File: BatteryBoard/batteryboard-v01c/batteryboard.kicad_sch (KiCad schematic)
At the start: 29 parts, among them J1 KEYSTONE-1042, J2 KEYSTONE-1042, J3 KEYSTONE-1042, J4 KEYSTONE-1042, J5 KEYSTONE-1042, J6 KEYSTONE-1042, J7 5023520601, J8 Screw_Terminal_01x02, Q1 IRF7458, Q2 IRF7458, Q3 MMBT2222AT, U1 R5460N233AF

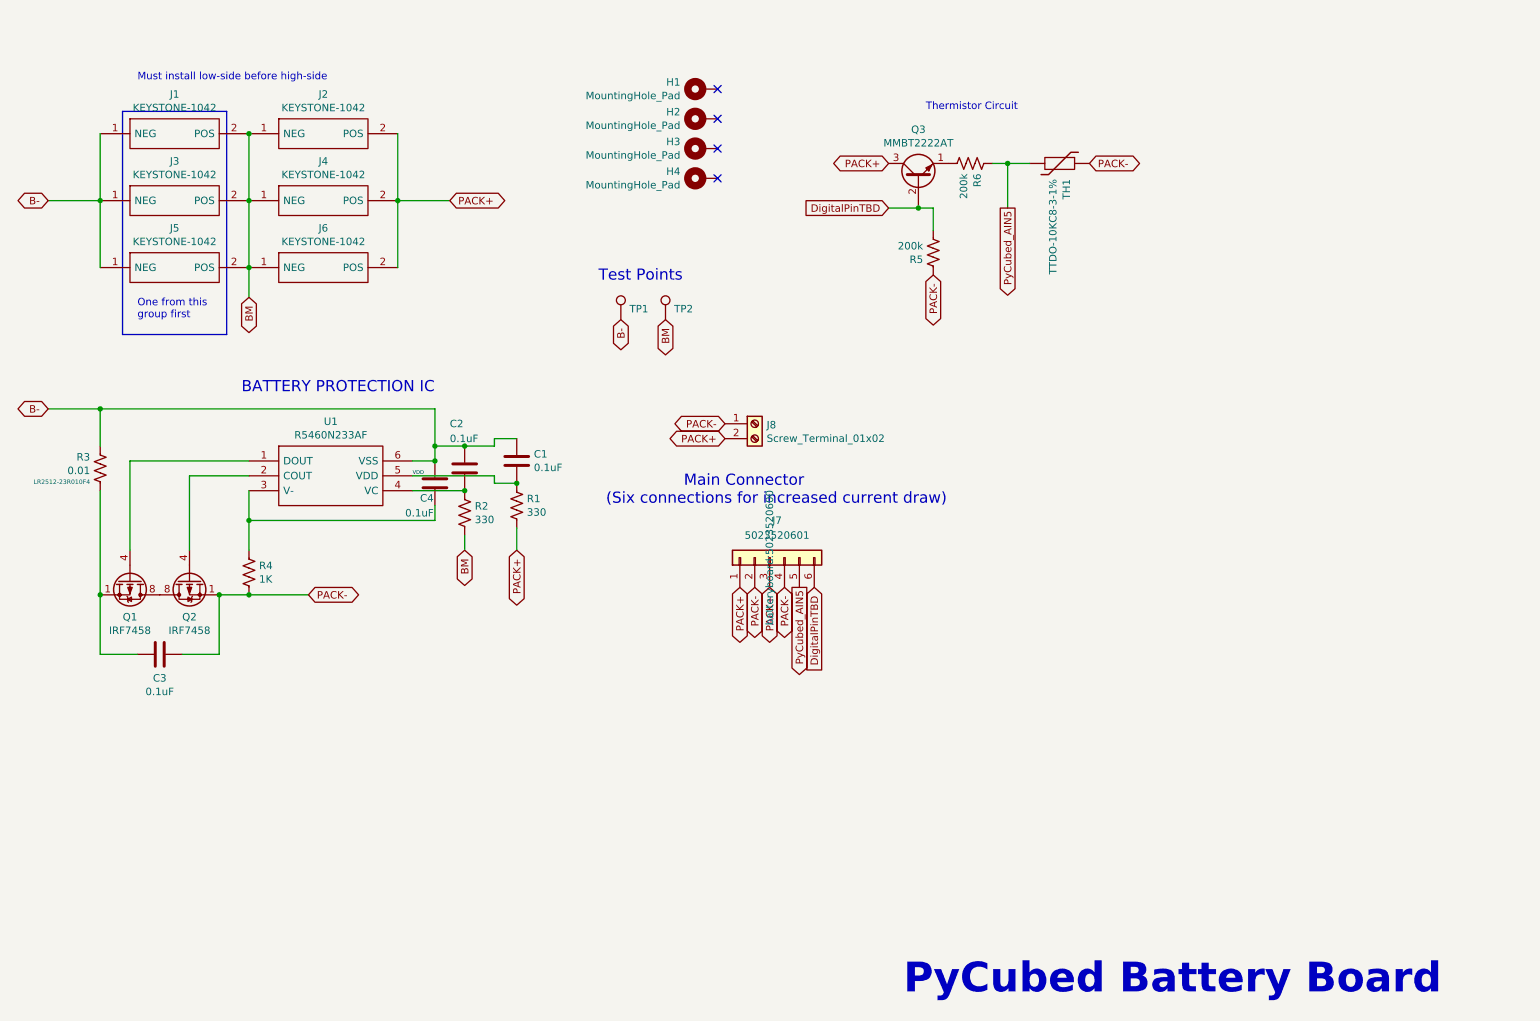
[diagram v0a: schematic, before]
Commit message: Added Sapling Files
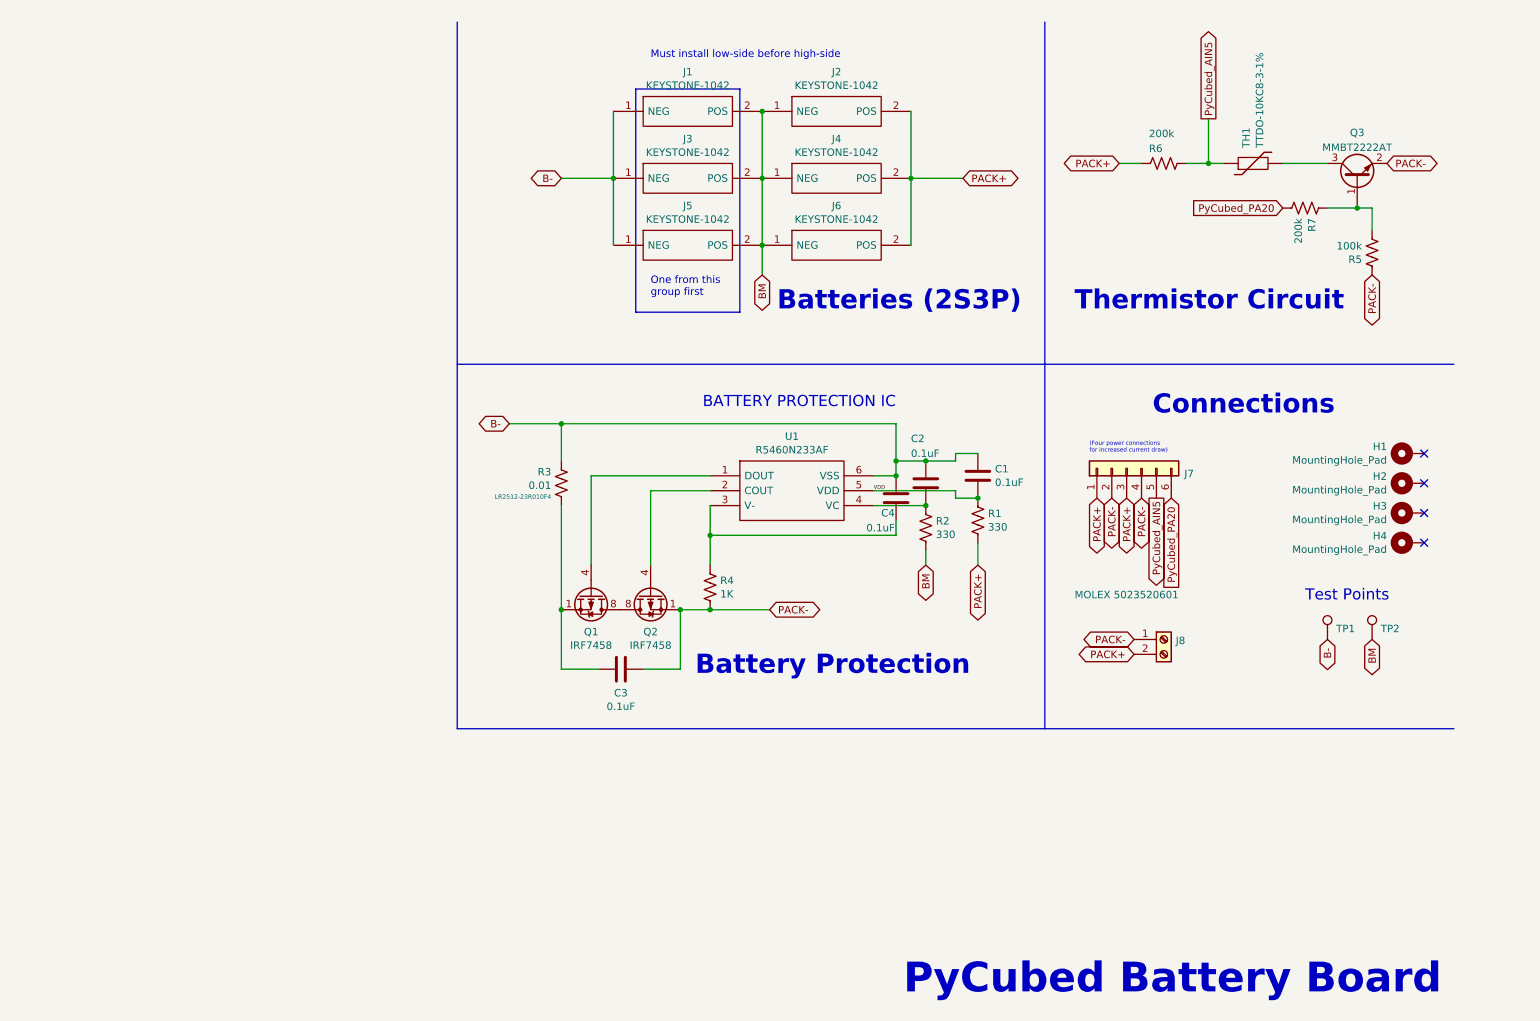
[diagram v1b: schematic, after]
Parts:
- removed Q3: MMBT2222AT, Package_TO_SOT_THT:TO-39-3, symbol Transistor_BJT:2N2219
- added Q3: MMBT2222AT, Package_TO_SOT_SMD:SOT-23, symbol Transistor_BJT:MMBT5551L
- added R7: 200k, Resistor_SMD:R_0603_1608Metric, symbol Device:R_US
- J1, J2, J3, J4, J5, J6: symbol batteryboard-rescue:1042-symbols -> batteryboard-rescue:1042-symbols-batteryboard-rescue
- J7: value 5023520601 -> MOLEX 5023520601
- R5: value 200k -> 100k
- R6: footprint Resistor_SMD:R_0603_1608Metric -> Resistor_SMD:R_1206_3216Metric
- U1: symbol batteryboard-rescue:R5460N233AF-symbols -> batteryboard-rescue:R5460N233AF-symbols-batteryboard-rescue
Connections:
- net PACK+: now also R6.1
- net PACK-: now also Q3.2 (E); no longer TH1.1
- net PyCubed_AIN5: now also TH1.1; no longer TH1.2
- net DigitalPinTBD: no longer names the net of R5.1
- net DigitalPinTBD: now also Q3.1 (B), R7.2; no longer J7.6 (Pin_6)
- new net: Q3.3 (C), TH1.2
- new net PyCubed_PA20: J7.6 (Pin_6), R7.1
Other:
- note added: "(Four power connections for increased current draw)"
- note added: "Batteries (2S3P)"
- note added: "Battery Protection"
- note added: "Connections"
- note removed: "Main Connector (Six connections for increased current draw)"
- moved on the sheet: C1, C2, C3, C4, H1, H2, H3, H4, J1, J2, J3, J4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
